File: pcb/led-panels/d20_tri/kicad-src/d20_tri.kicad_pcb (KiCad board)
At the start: 4 copper layers, 36.3 x 31.7 mm, 152 parts, among them J1 input, J2 output, Q1 LP0404N3T5G, Q10 LP0404N3T5G, Q11 LP0404N3T5G, Q12 LP0404N3T5G, Q13 LP0404N3T5G, Q14 LP0404N3T5G, Q15 LP0404N3T5G, Q2 LP0404N3T5G, Q3 LP0404N3T5G, Q4 LP0404N3T5G, Q5 LP0404N3T5G, Q6 LP0404N3T5G, Q7 LP0404N3T5G, Q8 LP0404N3T5G, Q9 LP0404N3T5G, U1 TLC59025, U2 TLC59025, U3 TLC59025, U4 74HC595, U5 74HC595, U6 NC7WZ17, U7 NC7WZ17

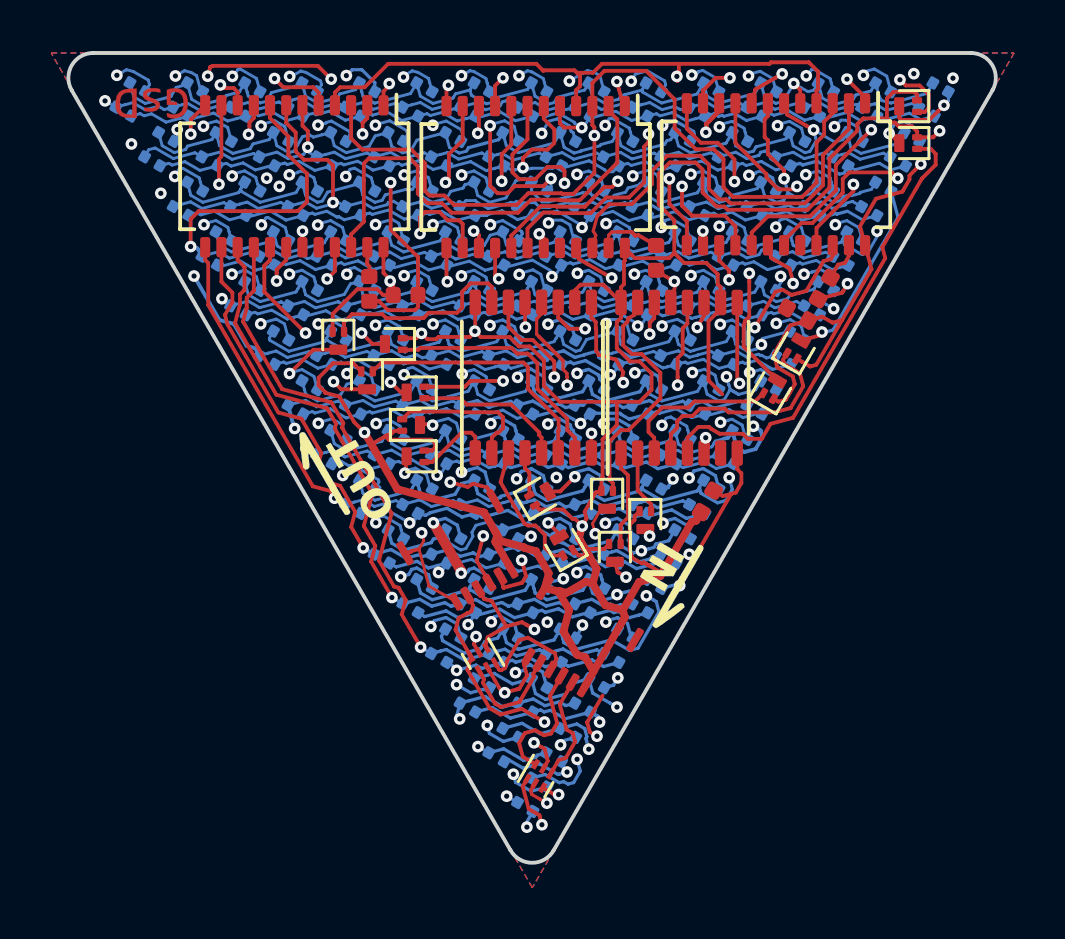
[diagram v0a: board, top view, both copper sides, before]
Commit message: Add and replace files from r1.0
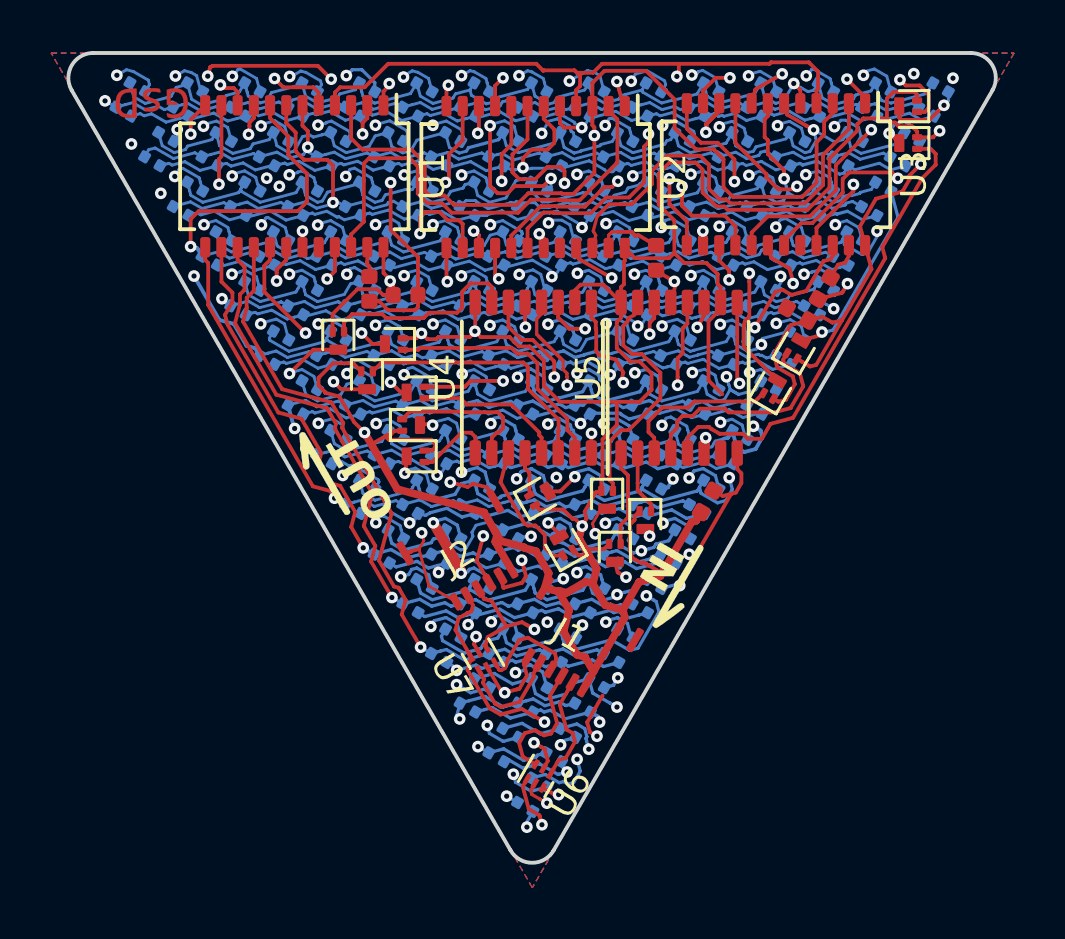
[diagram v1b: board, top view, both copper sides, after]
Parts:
- C1, C2, C3: value 100nF -> 470nF
- D1, D10, D100, D101, D102, D103, D104, D105, D11, D113, D114, D115, D116, D117, D118, D119, D12, D120, D129, D13, D130, D131, D132, D133, D134, D135, D14, D145, D146, D147, D148, D149, D15, D150, D161, D162, D163, D164, D165, D17, D177, D178, D179, D18, D180, D19, D193, D194, D195, D2, D20, D209, D21, D210, D22, D225, D23, D24, D25, D26, D27, D28, D29, D3, D30, D33, D34, D35, D36, D37, D38, D39, D4, D40, D41, D42, D43, D44, D45, D49, D5, D50, D51, D52, D53, D54, D55, D56, D57, D58, D59, D6, D60, D65, D66, D67, D68, D69, D7, D70, D71, D72, D73, D74, D75, D8, D81, D82, D83, D84, D85, D86, D87, D88, D89, D9, D90, D97, D98, D99: footprint gkl_led:led_rbag_1515 -> Led_Panel:LED_1515_RBGA_slim
- J1, J2: footprint gkl_conn:5034800600 -> Led_Panel:5034800600
- U1, U2, U3: footprint gkl_misc:SSOP-24_slim -> Led_Panel:SSOP-24_slim
- U4, U5: footprint gkl_misc:TSSOP-16_slim -> Led_Panel:TSSOP-16_slim
- U6, U7: footprint gkl_misc:UDFN-6_1x1mm_P0.35mm -> Led_Panel:UDFN-6_1x1mm_P0.35mm
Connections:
- J1 pad SH: vcc -> gnd
- U1 pad 20: colr_15 -> (no net)
- U2 pad 20: colg_15 -> (no net)
- U3 pad 20: colb_15 -> (no net)
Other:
- net class Default removed
- board text removed: "1"
- board text removed: "105"
- board text removed: "113"
- board text removed: "121"
- board text removed: "17"
- board text removed: "25"
- board text removed: "33"
- board text removed: "41"
- board text removed: "49"
- board text removed: "57"
- board text removed: "65"
- board text removed: "73"
- board text removed: "81"
- board text removed: "89"
- board text removed: "9"
- board text removed: "97"
